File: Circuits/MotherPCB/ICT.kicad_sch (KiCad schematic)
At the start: 1 part, among them J4 PINHD_1x4_Male

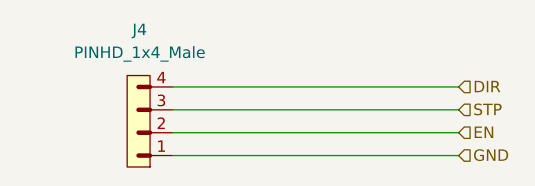
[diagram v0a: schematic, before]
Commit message: Schematic Finished
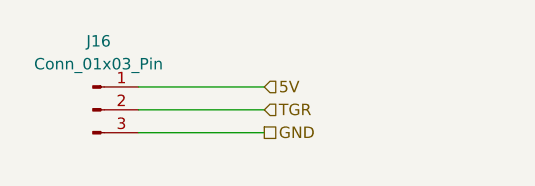
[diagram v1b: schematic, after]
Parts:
- removed J4: PINHD_1x4_Male, Connector_PinHeader_2.54mm:PinHeader_1x04_P2.54mm_Vertical, symbol PCM_SL_Pin_Headers:PINHD_1x4_Male
- added J16: Conn_01x03_Pin, symbol Connector:Conn_01x03_Pin
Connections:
- net GND: now also J16.3 (Pin_3)
- new net 5V: J16.1 (Pin_1)
- new net TGR: J16.2 (Pin_2)
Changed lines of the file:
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@@
 	(wire
 		(pts
-			(xy 121.92 102.87) (xy 153.67 102.87)
+			(xy 118.11 97.79) (xy 132.08 97.79)
 		)
 		(stroke
@@
 	(wire
 		(pts
-			(xy 121.92 97.79) (xy 153.67 97.79)
+			(xy 118.11 95.25) (xy 132.08 95.25)
 		)
 		(stroke
@@
 	(wire
 		(pts
-			(xy 121.92 100.33) (xy 153.67 100.33)
+			(xy 118.11 100.33) (xy 132.08 100.33)
 		)
 		(stroke
@@
 		)
 	)
-	(wire
-		(pts
-			(xy 121.92 95.25) (xy 153.67 95.25)
-		)
-		(stroke
-			(width 0)
-			(type default)
-		)
-	)
-	(hierarchical_label "STP"
+	(hierarchical_label "TGR"
 		(shape input)
-		(at 153.67 97.79 0)
-		(effects
-			(font
-				(size 1.27 1.27)
-			)
-			(justify left)
-		)
-	)
-	(hierarchical_label "DIR"
-		(shape input)
-		(at 153.67 95.25 0)
-		(effects
-			(font
-				(size 1.27 1.27)
-			)
-			(justify left)
-		)
-	)
-	(hierarchical_label "EN"
-		(shape input)
-		(at 153.67 100.33 0)
+		(at 132.08 97.79 0)
 		(effects
 			(font
@@
 	)
 	(hierarchical_label "GND"
+		(shape passive)
+		(at 132.08 100.33 0)
+		(effects
+			(font
+				(size 1.27 1.27)
+			)
+			(justify left)
+		)
+	)
+	(hierarchical_label "5V"
 		(shape input)
-		(at 153.67 102.87 0)
+		(at 132.08 95.25 0)
 		(effects
 			(font
@@
 	)
 	(symbol
-		(lib_id "PCM_SL_Pin_Headers:PINHD_1x4_Male")
-		(at 118.11 99.06 180)
+		(lib_id "Connector:Conn_01x03_Pin")
+		(at 113.03 97.79 0)
 		(unit 1)
 		(exclude_from_sim no)
@@
 		(dnp no)
 		(fields_autoplaced yes)
-		(property "Reference" "J4"
-			(at 118.235 88.9 0)
+		(property "Reference" "J16"
+			(at 113.665 90.17 0)
 			(effects
 				(font
@@
 			)
 		)
-		(property "Value" "PINHD_1x4_Male"
-			(at 118.235 91.44 0)
+		(property "Value" "Conn_01x03_Pin"
+			(at 113.665 92.71 0)
 			(effects
 				(font
@@
 			)
 		)
-		(property "Footprint" "Connector_PinHeader_2.54mm:PinHeader_1x04_P2.54mm_Vertical"
-			(at 119.38 110.49 0)
+		(property "Footprint" ""
+			(at 113.03 97.79 0)
 			(effects
 				(font
@@
 			)
 		)
-		(property "Datasheet" ""
-			(at 118.11 109.22 0)
+		(property "Datasheet" "~"
+			(at 113.03 97.79 0)
 			(effects
 				(font
@@
 			)
 		)
-		(property "Description" "Pin Header male with pin space 2.54mm. Pin Count -4"
-			(at 118.11 99.06 0)
+		(property "Description" "Generic connector, single row, 01x03, script generated"
+			(at 113.03 97.79 0)
 			(effects
 				(font
@@
 		(pin "2"
 		)
-		(pin "4"
-		)
 		(instances
 			(project ""
 				(path "/ea485091-218e-4ddf-97d6-ebaac999a2f0/60749f9c-7a77-4668-8fdc-88ae42547d8b"
-					(reference "J4")
+					(reference "J16")
 					(unit 1)
 				)

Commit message: Fixed some broken footprints
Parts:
- J16: footprint (none) -> Connector_PinHeader_2.54mm:PinHeader_1x03_P2.54mm_Vertical
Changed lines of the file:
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@@
 			)
 		)
-		(property "Footprint" ""
+		(property "Footprint" "Connector_PinHeader_2.54mm:PinHeader_1x03_P2.54mm_Vertical"
 			(at 113.03 97.79 0)
 			(effects
